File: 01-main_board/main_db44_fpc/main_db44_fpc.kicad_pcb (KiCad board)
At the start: 4 copper layers, 62 x 38 mm, 4 parts, among them J1 DB44_Female

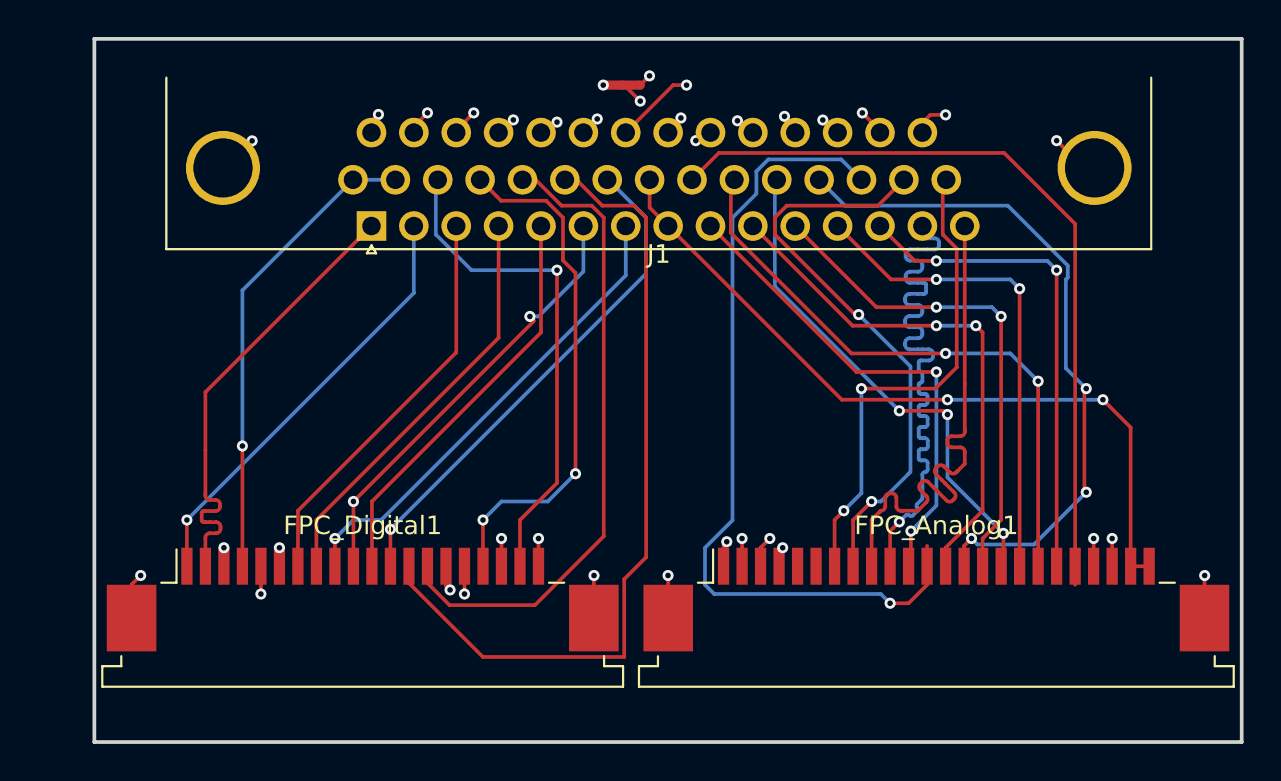
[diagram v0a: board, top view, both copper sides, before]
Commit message: update db44
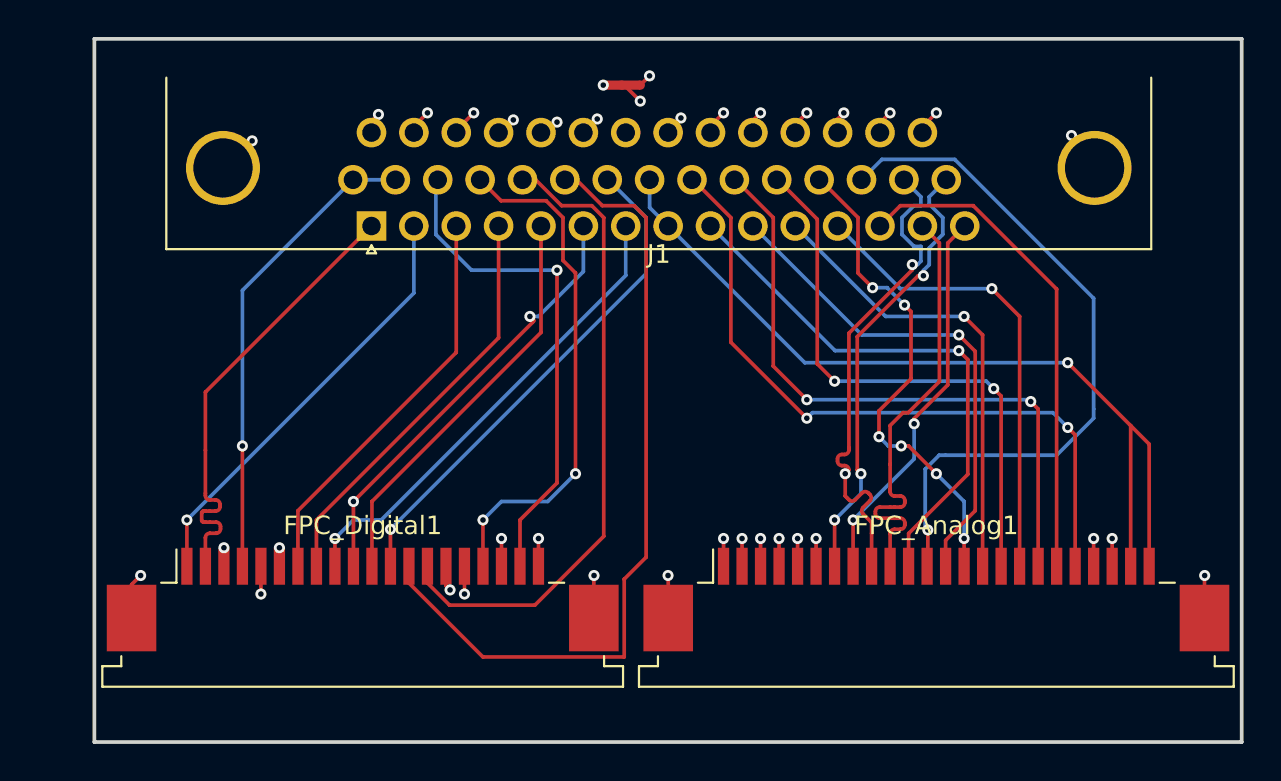
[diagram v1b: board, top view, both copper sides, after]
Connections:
- net sg_kelvin_2_FR renamed sg_sense_2_FR-
- net sg_sense_1_FL renamed sg_sense_1_FL+
- FPC_Analog1 pad 8: sg_kelvin_1_FL -> sg_sense_1_FL-
- FPC_Analog1 pad 9: sg_sense_2_FR -> sg_sense_2_FR+
- J1 pad 15: sg_sense_2_FR -> sg_sense_1_FL-
- J1 pad 29: sg_kelvin_1_FL -> sg_sense_2_FR+
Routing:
- net sg_kelvin_1_FL: track 31.4 -> 0.00 mm, vias 2 -> 0
- net sg_sense_2_FR: track 29.2 -> 0.00 mm
- net sg_sense_2_FR+: track 0.00 -> 27.3 mm, vias 0 -> 2
- net sg_sense_1_FL-: track 0.00 -> 20.9 mm, vias 0 -> 2
- net AN7: track 37.4 -> 26.7 mm, vias 3 -> 6
- net sg_sense_1_FL+: track 32.6 -> 23.9 mm, vias 1 -> 0
- net 11V1: track 40.9 -> 48.0 mm, vias 2 -> 1
- net AN6: track 44.8 -> 38.2 mm
- net AN10: track 42.4 -> 37.7 mm, vias 0 -> 2
- net B-: track 6.55 -> 2.21 mm, vias 3 -> 2
- net AN8: track 27.9 -> 30.7 mm, vias 3 -> 2
- net AN5: track 26.6 -> 29.4 mm, vias 2 -> 1
- net sg_sense_2_FR-: track 26.4 -> 24.3 mm, vias 2 -> 3
- net AN3: track 27.1 -> 25.1 mm, vias 2 -> 1
- net AN9: track 32.9 -> 34.7 mm
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
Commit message: Added comments
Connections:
- J1 pad 0: GNDA -> GNDD
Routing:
- net GNDD: track 16.3 -> 18.5 mm, vias 12 -> 13
- net GNDA: track 21.5 -> 19.4 mm, vias 13 -> 12
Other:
- board text added: "NOT a right angle connector"
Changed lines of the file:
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@@
 			(layers "*.Cu" "*.Mask")
 			(remove_unused_layers no)
-			(net 4 "GNDA")
+			(net 20 "GNDD")
 			(pinfunction "MH")
 			(pintype "passive")
@@
 		(layer "Edge.Cuts")
 	)
+	(gr_text "NOT a right angle connector"
+		(at 184.5 68.5 0)
+		(layer "Cmts.User")
+		(effects
+			(font
+				(size 1 1)
+				(thickness 0.15)
+			)
+			(justify left bottom)
+		)
+	)
+	(dimension
+		(type orthogonal)
+		(layer "Cmts.User")
+		(pts
+			(xy 124.5 109.5) (xy 186.5 109.5)
+		)
+		(height 8)
+		(orientation 0)
+		(format
+			(prefix "")
+			(suffix "")
+			(units 3)
+			(units_format 0)
+			(precision 4)
+			(suppress_zeroes yes)
+		)
+		(style
+			(thickness 0.1)
+			(arrow_length 1.27)
+			(text_position_mode 0)
+			(arrow_direction outward)
+			(extension_height 0.58642)
+			(extension_offset 0.5)
+			(keep_text_aligned yes)
+		)
+		(gr_text "62"
+			(at 155.5 116.35 0)
+			(layer "Cmts.User")
+			(effects
+				(font
+					(size 1 1)
+					(thickness 0.15)
+				)
+			)
+		)
+	)
+	(dimension
+		(type orthogonal)
+		(layer "Cmts.User")
+		(pts
+			(xy 124.5 71.5) (xy 124.5 109.5)
+		)
+		(height -21.5)
+		(orientation 1)
+		(format
+			(prefix "")
+			(suffix "")
+			(units 3)
+			(units_format 0)
+			(precision 4)
+			(suppress_zeroes yes)
+		)
+		(style
+			(thickness 0.1)
+			(arrow_length 1.27)
+			(text_position_mode 0)
+			(arrow_direction outward)
+			(extension_height 0.58642)
+			(extension_offset 0.5)
+			(keep_text_aligned yes)
+		)
+		(gr_text "38"
+			(at 101.85 90.5 90)
+			(layer "Cmts.User")
+			(effects
+				(font
+					(size 1 1)
+					(thickness 0.15)
+				)
+			)
+		)
+	)
 	(segment
 		(start 173 85)
@@
 	)
 	(segment
-		(start 131.45 78.475)
-		(end 132.91297 77.01203)
-		(width 0.2)
-		(layer "F.Cu")
-		(net 4)
-	)
-	(segment
 		(start 178.55 78.475)
 		(end 178.55 77.970321)
@@
 	)
 	(segment
-		(start 132.91297 77.01203)
-		(end 133.025506 77.01203)
-		(width 0.2)
-		(layer "F.Cu")
-		(net 4)
-	)
-	(segment
 		(start 153.136 74)
 		(end 154 74.864)
@@
 	(via
 		(at 184.5 100.5)
-		(size 0.6)
-		(drill 0.3)
-		(layers "F.Cu" "B.Cu")
-		(net 4)
-	)
-	(via
-		(at 133.025506 77.01203)
 		(size 0.6)
 		(drill 0.3)
@@
 	)
 	(segment
+		(start 131.45 78.475)
+		(end 132.91297 77.01203)
+		(width 0.2)
+		(layer "F.Cu")
+		(net 20)
+	)
+	(segment
 		(start 134.5 100)
 		(end 134.5 99)
@@
 	)
 	(segment
+		(start 132.91297 77.01203)
+		(end 133.025506 77.01203)
+		(width 0.2)
+		(layer "F.Cu")
+		(net 20)
+	)
+	(segment
 		(start 144.5 100)
 		(end 144.5 101.5)
@@
 		(size 0.6)
 		(drill 0.3)
+		(layers "F.Cu" "B.Cu")
+		(net 20)
+	)
+	(via
+		(at 133.025506 77.01203)
+		(size 0.6)
+		(drill 0.3)

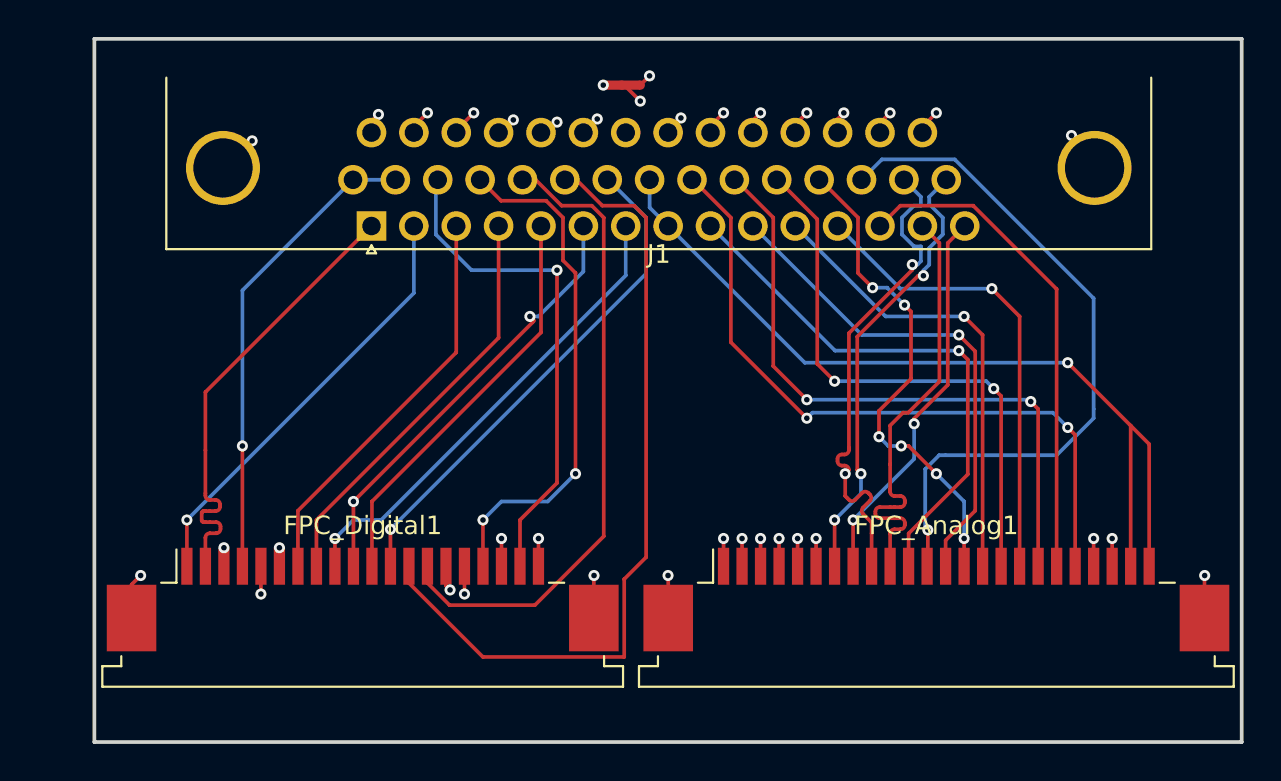
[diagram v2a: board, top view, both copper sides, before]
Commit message: update db44
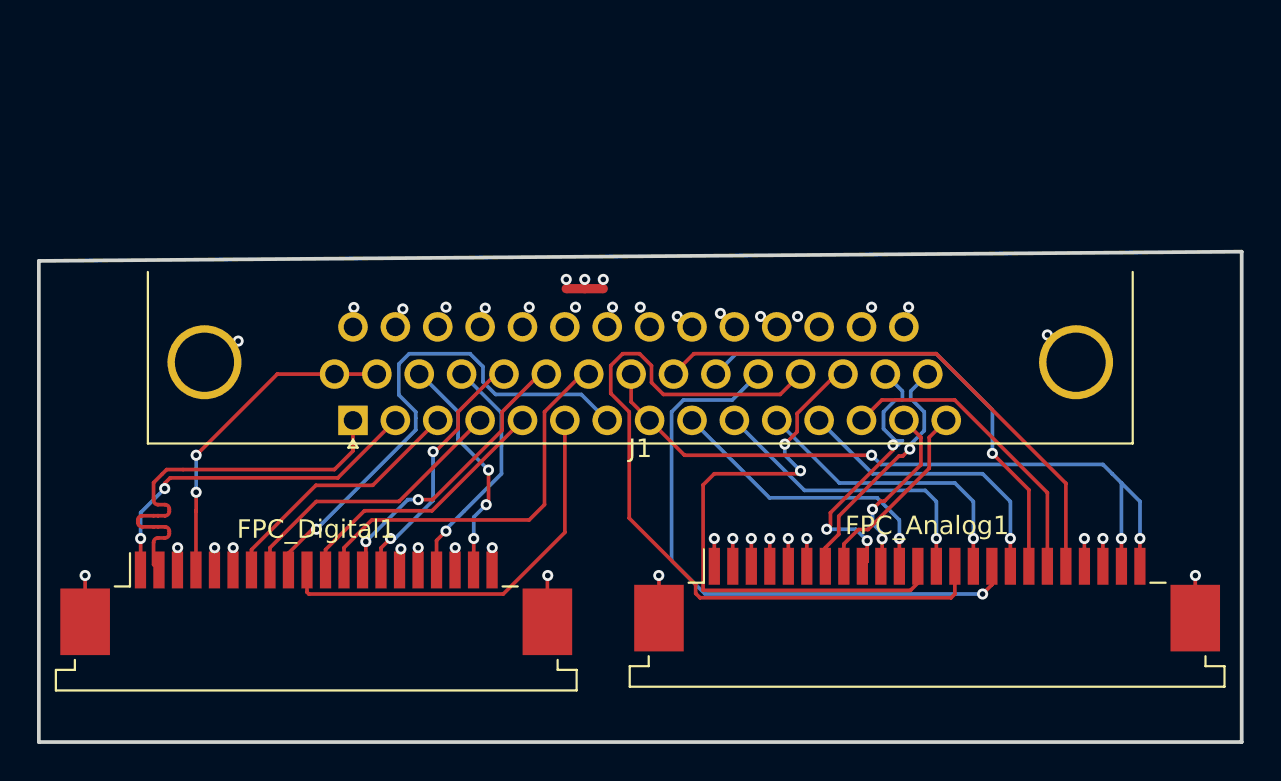
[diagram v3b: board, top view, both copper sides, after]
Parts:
- moved NT1 11.2 mm to (151.0, 85.0)
- moved J1 10.5 mm to (138.5, 90.9)
- moved FPC_Digital1 2.52 mm to (136.5, 102.0)
- moved FPC_Analog1 0.50 mm to (169.5, 101.8)
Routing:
- net D5: track 43.8 -> 15.7 mm, vias 0 -> 2
- net D6: track 34.9 -> 13.8 mm, vias 0 -> 2
- net AN7: track 26.7 -> 42.3 mm, vias 6 -> 0
- net GP/Int1: track 28.0 -> 13.0 mm, vias 2 -> 1
- net GP/Int2: track 27.2 -> 12.5 mm, vias 1 -> 3
- net sg_sense_1_FL+: track 23.9 -> 9.72 mm, vias 0 -> 2
- net AN5: track 29.4 -> 15.9 mm
- net sg_sense_2_FR+: track 27.3 -> 15.8 mm, vias 2 -> 3
- net AN4: track 27.1 -> 16.2 mm
- net sg_sense_2_FR-: track 24.3 -> 13.5 mm, vias 3 -> 1
- net sg_sense_1_FL-: track 20.9 -> 10.5 mm, vias 2 -> 0
- net AN1: track 26.8 -> 16.6 mm
- net AN2: track 25.4 -> 15.7 mm
- net AN3: track 25.1 -> 15.9 mm
- net AN9: track 34.7 -> 25.9 mm, vias 2 -> 1
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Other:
- board size 62 x 38 mm -> 65 x 26.5 mm
